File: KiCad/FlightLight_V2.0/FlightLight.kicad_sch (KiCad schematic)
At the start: 27 parts, among them J3 Conn_02x05_Odd_Even, SW1 AP, U2 ULN2003, U3 ESP-12F, U4 AMS1117-3.3

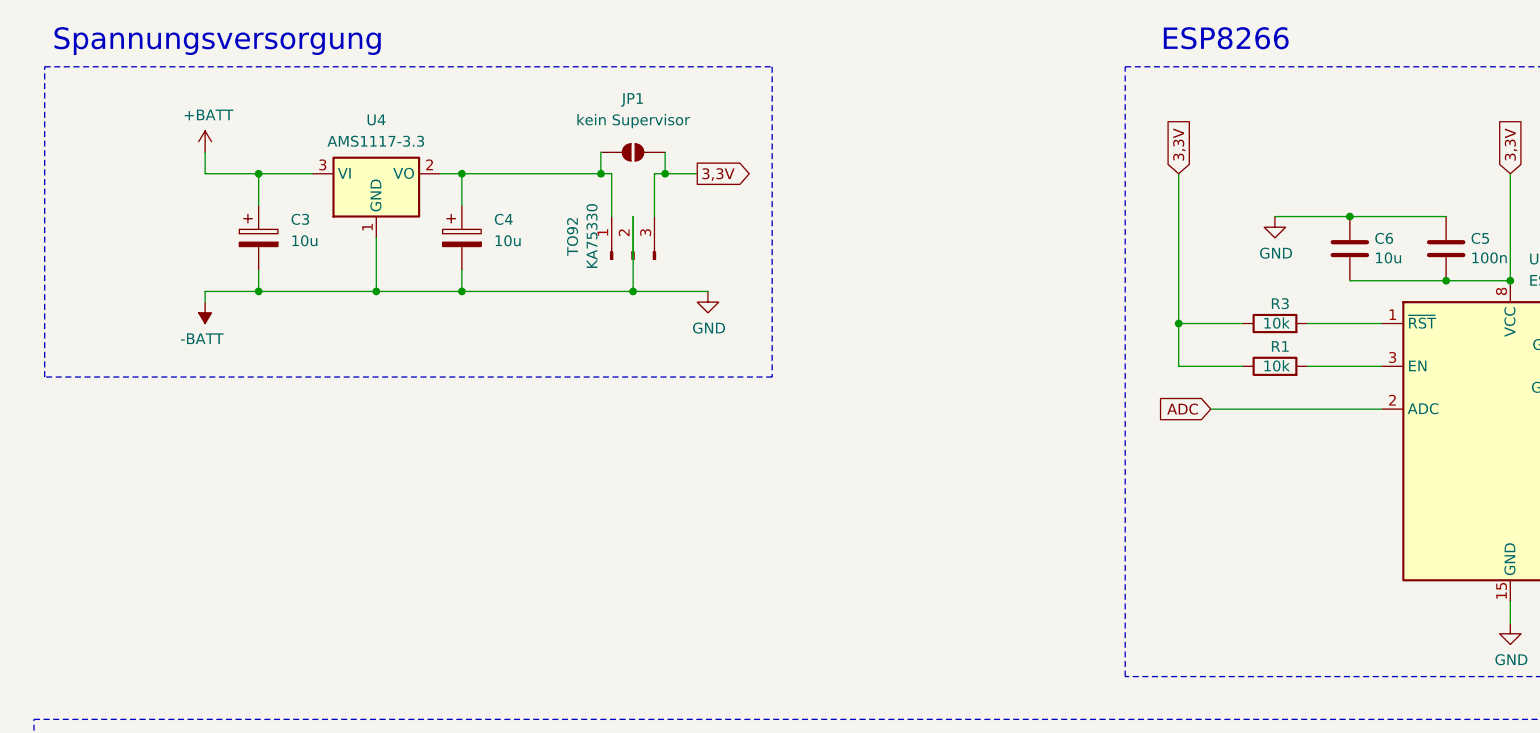
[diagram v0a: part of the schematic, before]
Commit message: PCB V2.1
kleine Fixes
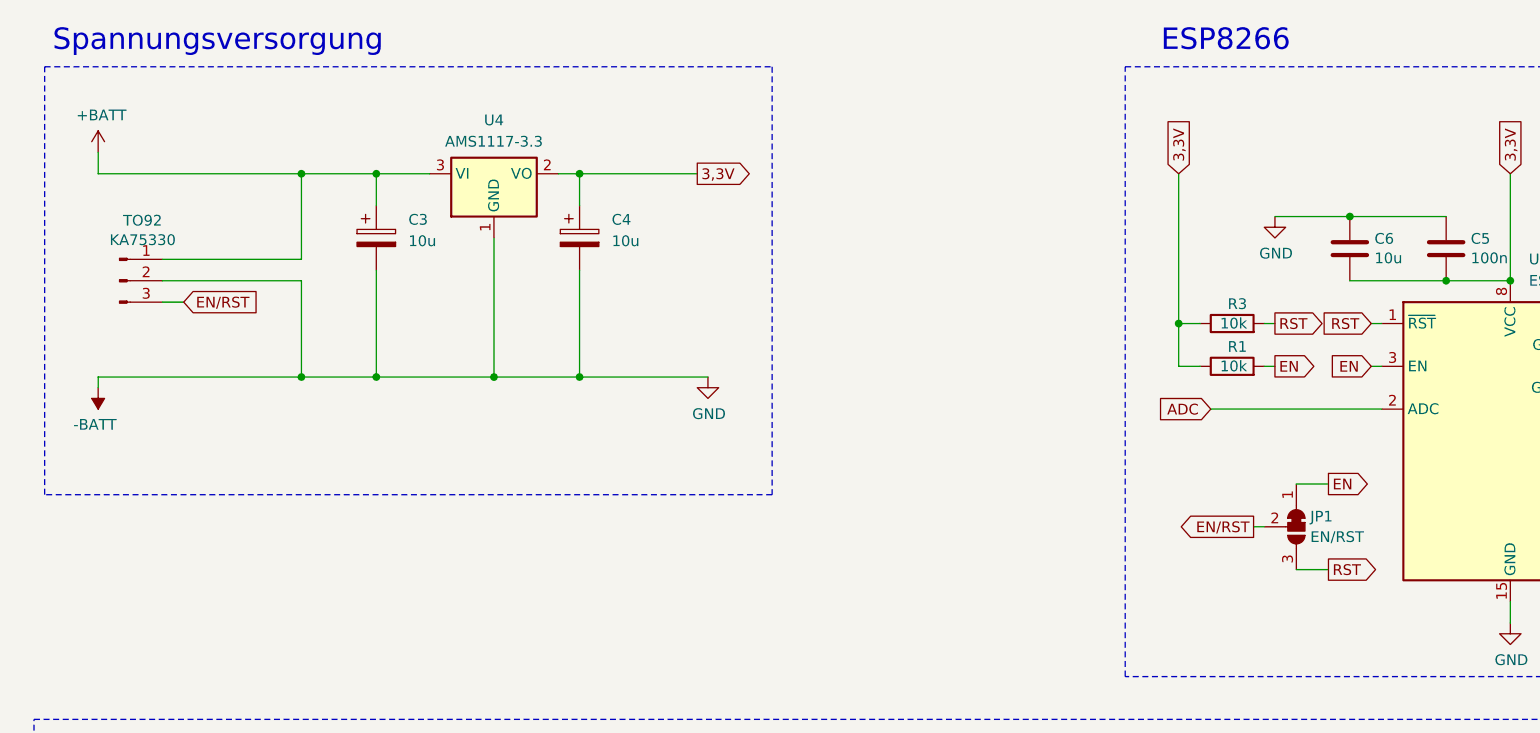
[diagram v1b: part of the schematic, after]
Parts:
- removed JP1: kein Supervisor, Jumper:SolderJumper-2_P1.3mm_Open_RoundedPad1.0x1.5mm, symbol Jumper:SolderJumper_2_Open
- added JP1: EN/RST, Jumper:SolderJumper-3_P1.3mm_Bridged12_RoundedPad1.0x1.5mm, symbol Jumper:SolderJumper_3_Bridged12
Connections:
- net +BATT: now also TO92.1 (Pin_1)
- net 3,3V: now also C4.1, U4.2 (VO); no longer TO92.3 (Pin_3)
- net RST: now reaches R3.2, U3.1 (~{RST})
- net RST: now also JP1.3 (B)
- net EN: now reaches R1.2, U3.3 (EN)
- net EN: now also JP1.1 (A)
- new net EN/RST: JP1.2 (C), TO92.3 (Pin_3)
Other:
- moved on the sheet: C3, C4, R1, R3, TO92, U4
